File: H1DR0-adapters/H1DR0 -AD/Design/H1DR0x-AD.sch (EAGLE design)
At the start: 3 parts

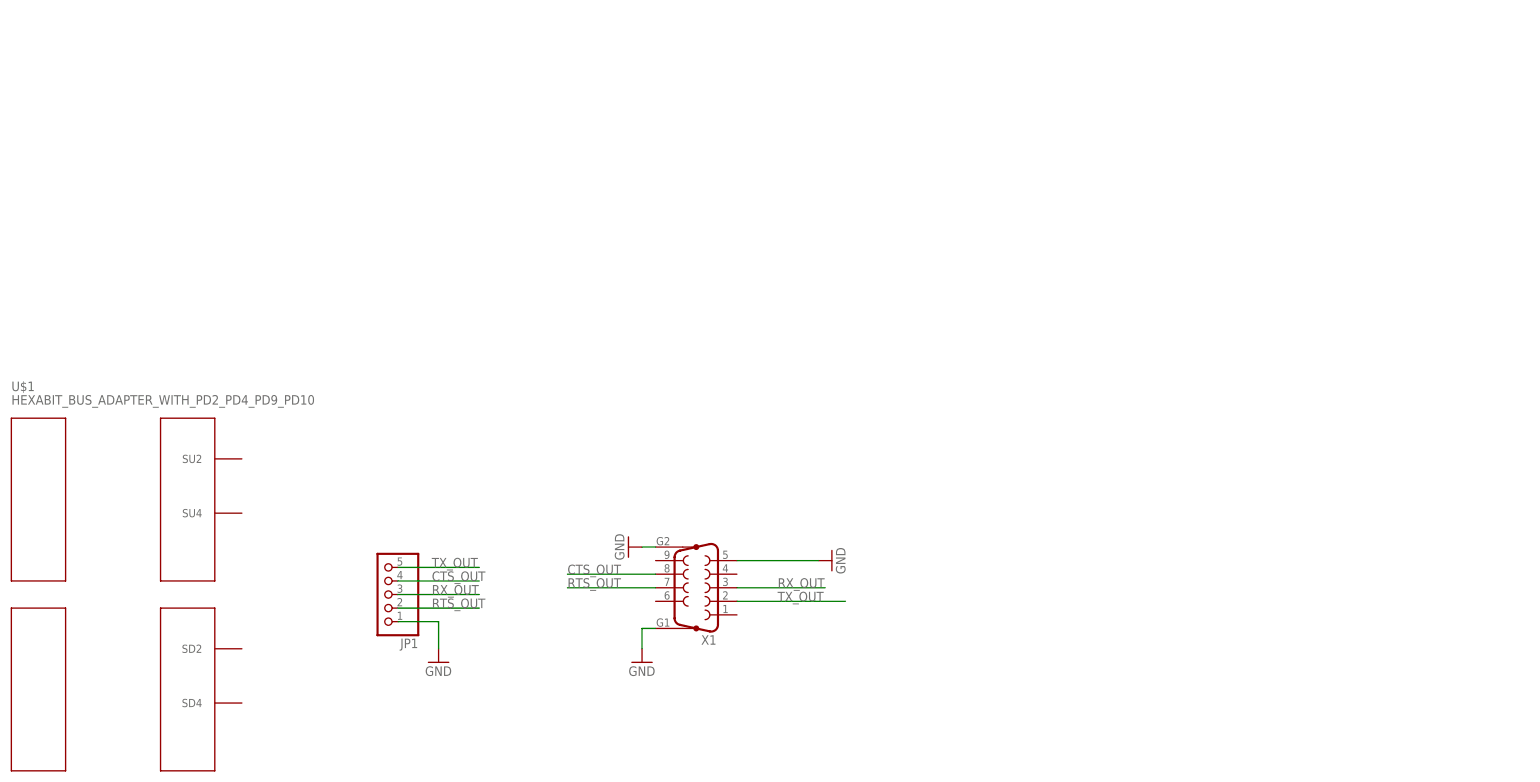
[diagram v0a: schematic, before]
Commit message: no message
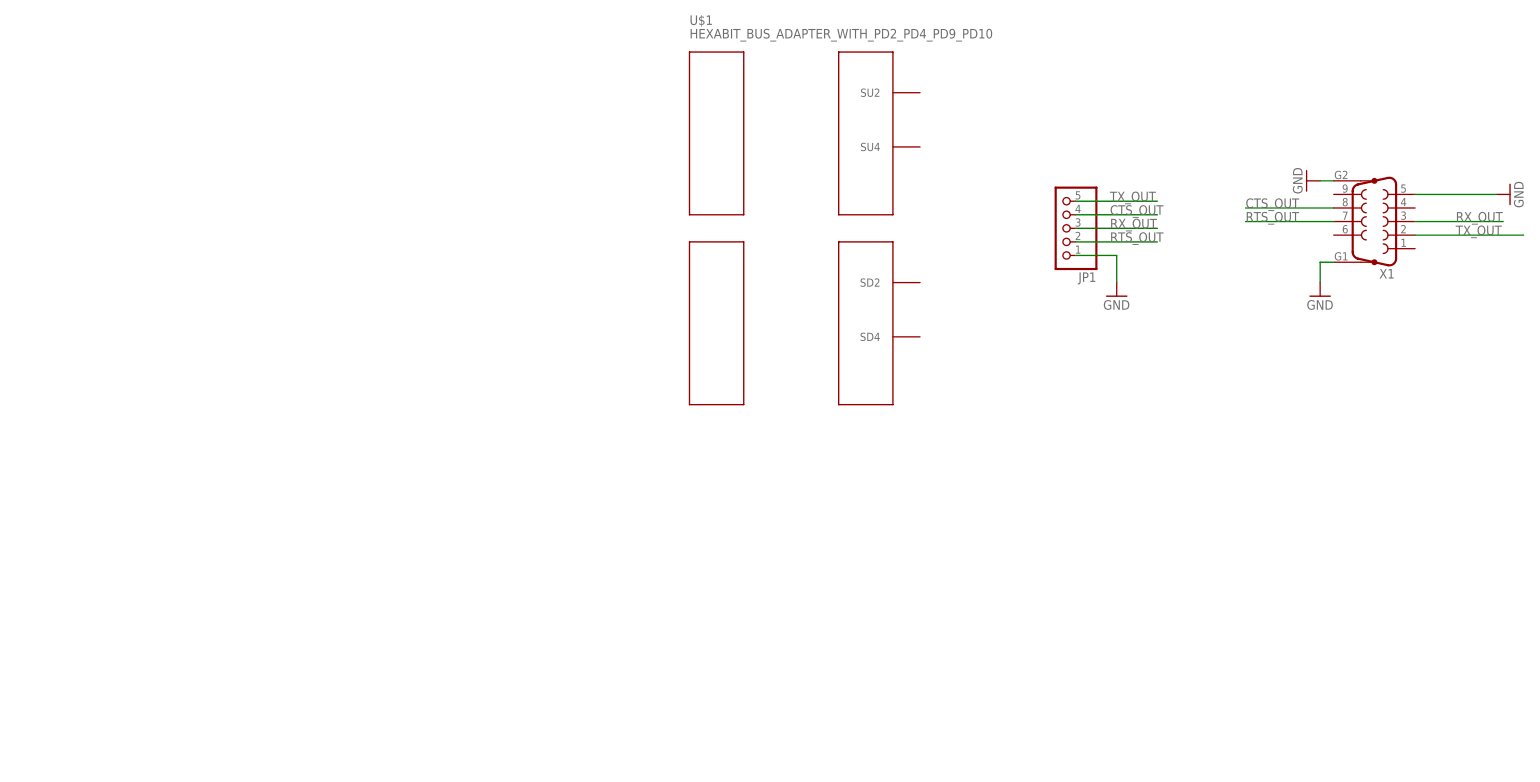
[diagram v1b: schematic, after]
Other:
- note added: "1"
- note added: "2"
- note added: "Amir Tabbakh"
- note added: "Author"
- note added: "DB9 adapter for H1DR0-AD"
- note added: "Description"
- note added: "H1DR0-AD"
- note added: "H1DR0-AD_Frontend"
- note added: "Letter"
- note added: "Module"
- note added: "Revision"
- note added: "Sheet of"
- note added: "Size"
- note added: "Title"
- note added: "www.hexabitz.com"
- note added: "z"
- moved on the sheet: JP1, U$1, X1
